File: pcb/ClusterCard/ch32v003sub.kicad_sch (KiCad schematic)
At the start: 3 parts

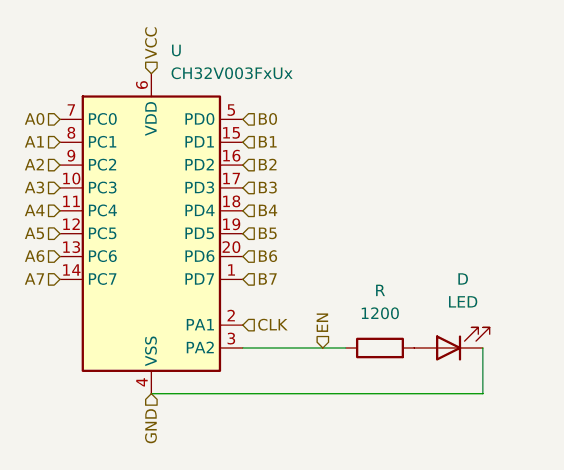
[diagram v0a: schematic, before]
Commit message: correct cluster card files
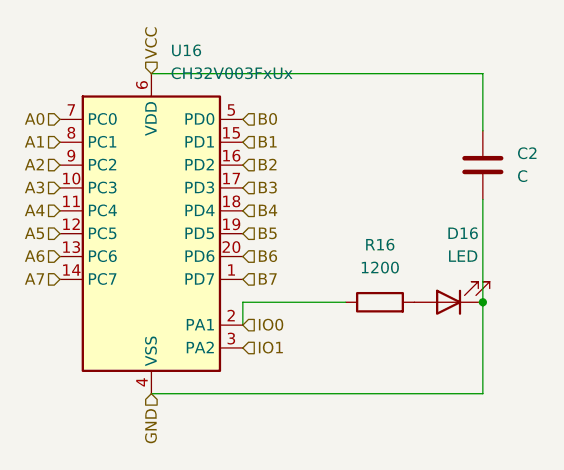
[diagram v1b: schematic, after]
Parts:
- added C2: C, Basics:C_0402_1005Metric, symbol Device:C
- D16: renamed from D; footprint (none) -> Basics:LED_0402_1005Metric
- R16: renamed from R; footprint (none) -> Basics:R_0402_1005Metric
- U16: renamed from U; footprint Package_DFN_QFN:QFN-20-1EP_3x3mm_P0.4mm_EP1.65x1.65mm -> Basics:QFN-20-1EP_3x3mm_P0.4mm_EP1.65x1.65mm_min
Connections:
- net GND: now also C2.2
- net VCC: now also C2.1
- net CLK renamed IO0
- net IO0: now also R16.1
- net EN renamed IO1
- net IO1: no longer R16.1
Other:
- moved on the sheet: D16, R16
